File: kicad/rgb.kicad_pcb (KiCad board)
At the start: 2 copper layers, 5 parts, among them Q1 DMG9926USD, Q2 DMG9926USD, Q3 DMG9926USD, Q4 DMG9926USD, U1 ATTINY404-SSNR

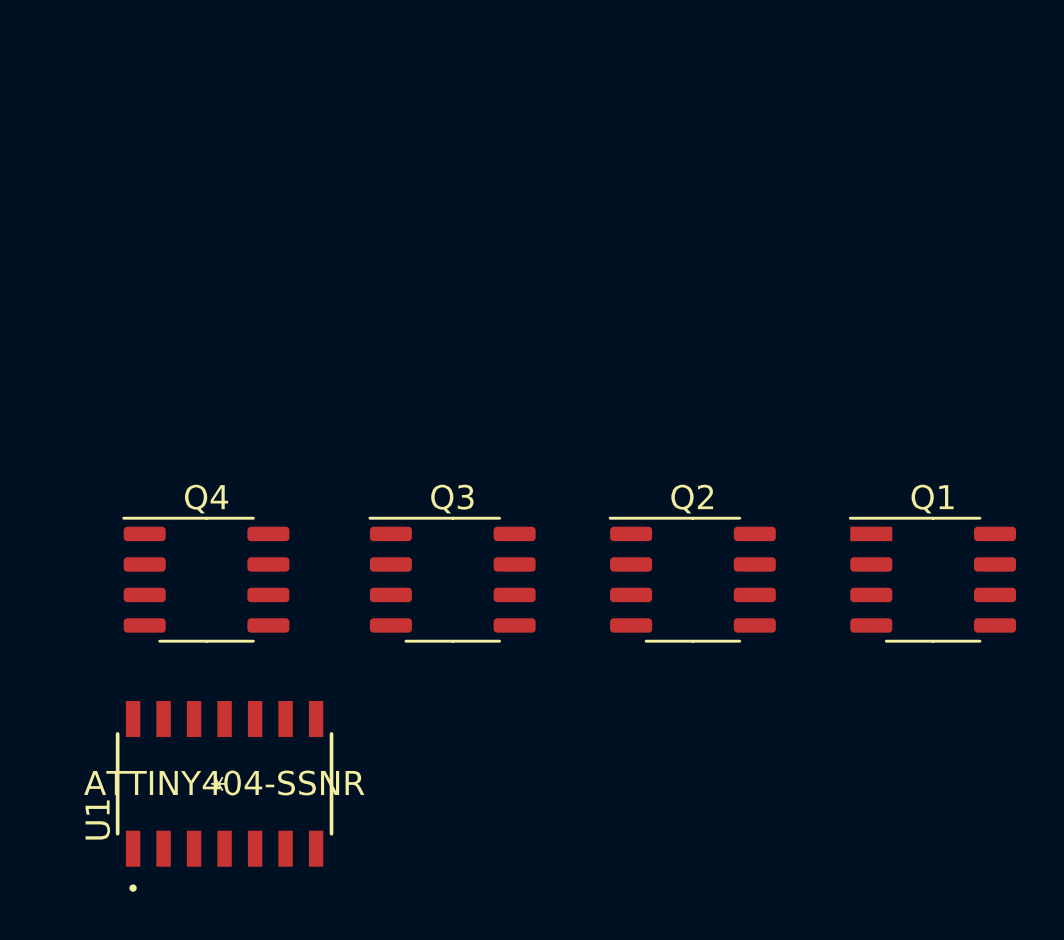
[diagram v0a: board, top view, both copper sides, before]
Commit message: ATTINY216
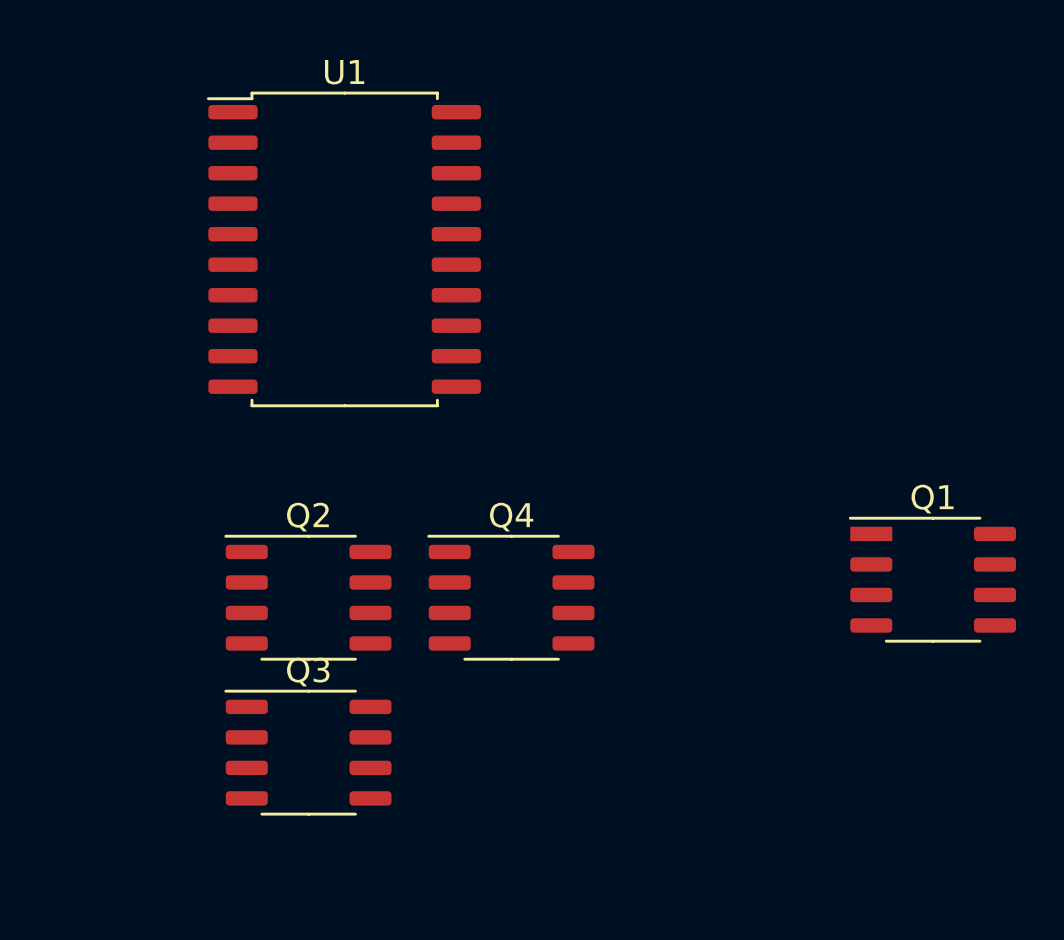
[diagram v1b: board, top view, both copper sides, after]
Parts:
- U1: value ATTINY404-SSNR -> ATtiny416-SNR; footprint rgb_footprints:ATTINY404-SSNR -> Package_SO:SOIC-20W_7.5x12.8mm_P1.27mm
- moved U1 22.8 mm to (171.8, 83.8), turned to 0 degrees
- moved Q2 16.0 mm to (170.2, 98.2)
- moved Q4 12.7 mm to (178.7, 98.2)
- moved Q3 9.37 mm to (170.2, 104.7)
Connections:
- Q1 pad 1: (no net) -> GND
- Q1 pad 2: (no net) -> /PWM_1
- Q1 pad 3: (no net) -> GND
- Q1 pad 4: (no net) -> /PWM_2
- Q2 pad 1: (no net) -> GND
- Q2 pad 2: (no net) -> /PWM_3
- Q2 pad 3: (no net) -> GND
- Q2 pad 4: (no net) -> /PWM_4
- Q3 pad 1: (no net) -> GND
- Q3 pad 3: (no net) -> GND
- Q4 pad 1: (no net) -> GND
- Q4 pad 2: (no net) -> /PWM_7
- Q4 pad 3: (no net) -> GND
- Q4 pad 4: (no net) -> /PWM_8
- U1 pad 10: (no net) -> /PWM_2
- U1 pad 11: (no net) -> /PWM_1
- U1 pad 12: (no net) -> /PWM_7
- U1 pad 13: (no net) -> /PWM_8
- U1 pad 9: (no net) -> /PWM_3
